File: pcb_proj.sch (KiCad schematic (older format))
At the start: 11 parts, among them U0 OPA333xxDBV, U1 OPA333xxDBV, U2 OPA333xxDBV, U3 OPA333xxDBV, U4 OPA333xxDBV, U5 OPA333xxDBV, U6 OPA333xxDBV, U7 OPA333xxDBV, U8 OPA333xxDBV, U9 OPA333xxDBV

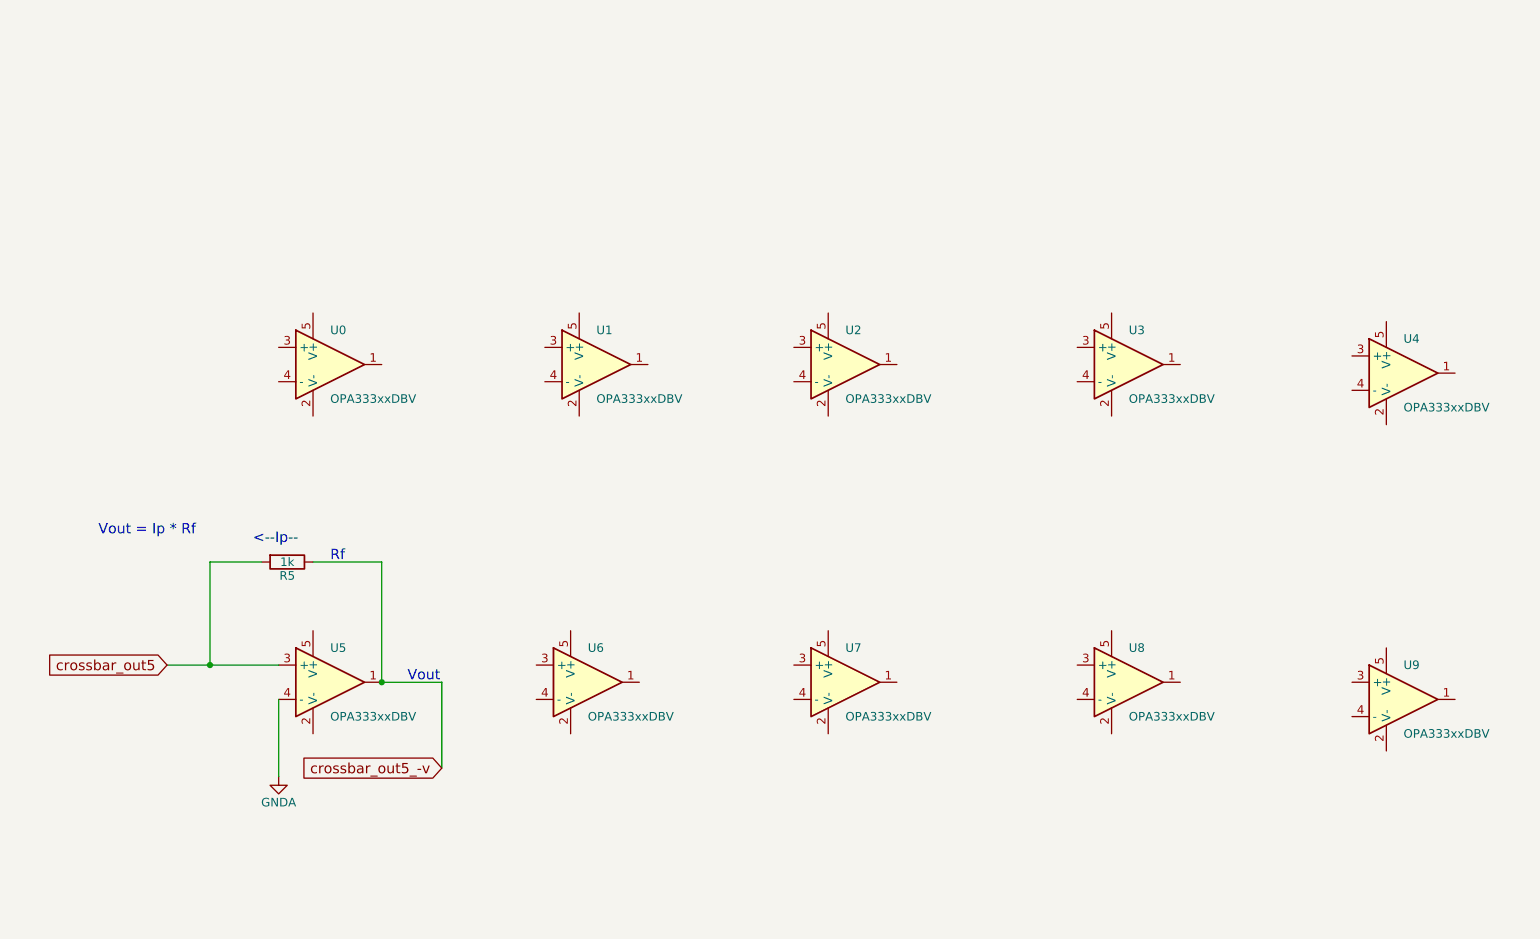
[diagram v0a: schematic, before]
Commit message: About to make a heirarchy, committing first in case we need to go back
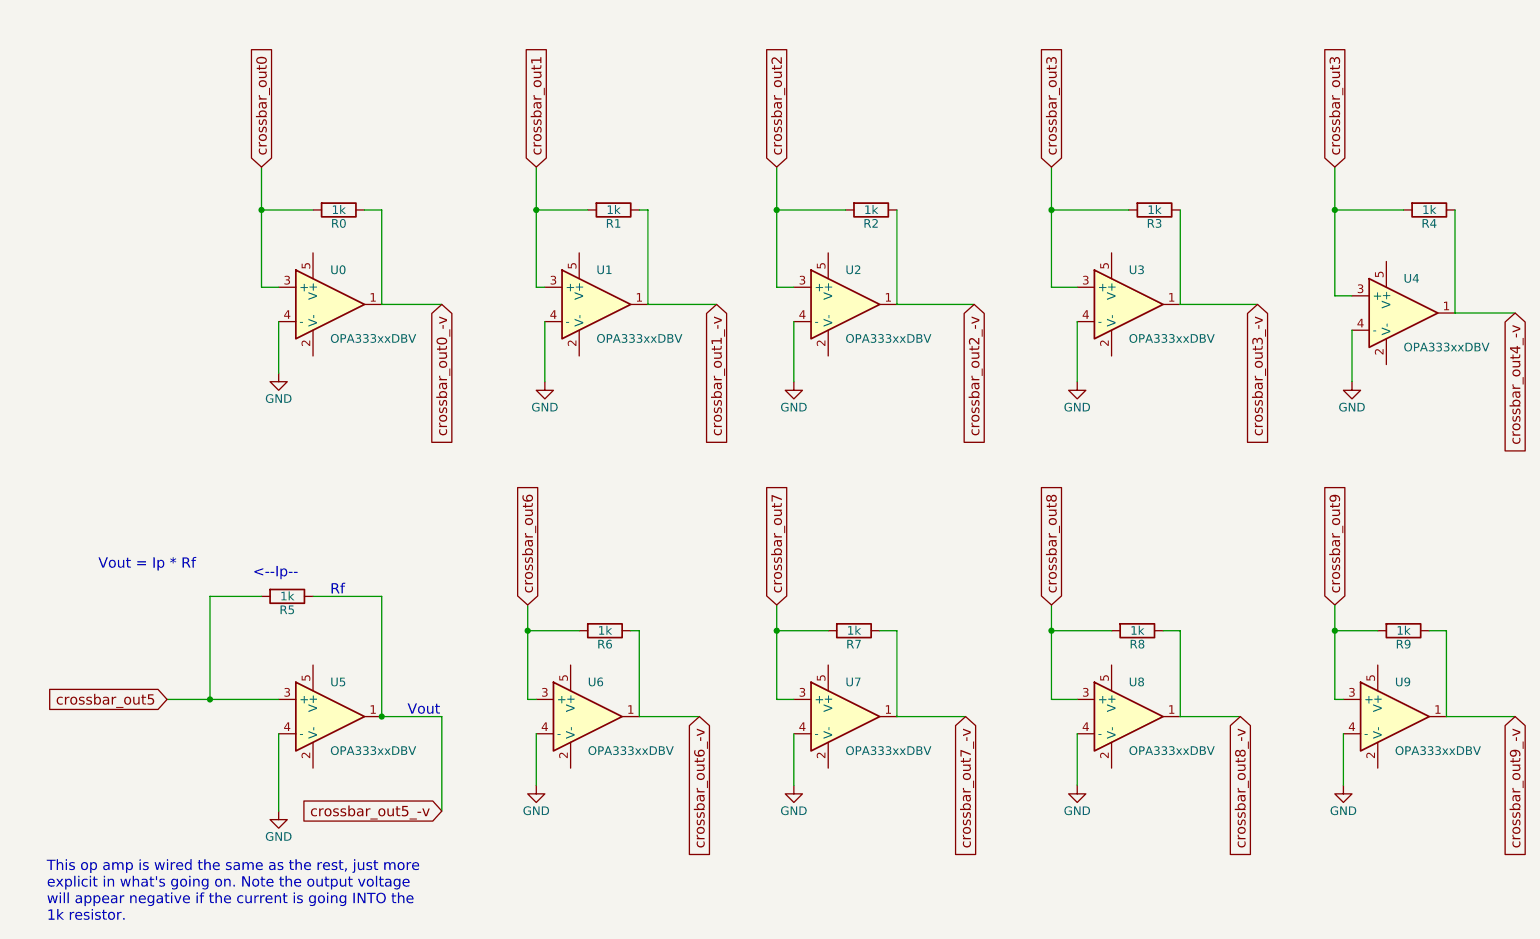
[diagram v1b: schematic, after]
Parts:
- added R0, R1, R2, R3, R4, R6, R7, R8, R9: 1k, symbol R
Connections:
- net GNDA is gone; now on net GND: U5.4 (-)
- net crossbar_out4_-v: now reaches U4.1
- net crossbar_out4_-v: now also R4.1
- net crossbar_out3: now reaches U4.3 (+)
- net crossbar_out3: now also U3.3 (+), R3.2, R4.2
- net GND: now reaches U4.4 (-)
- net GND: now also U0.4 (-), U1.4 (-), U2.4 (-), U3.4 (-), U6.4 (-), U7.4 (-), U8.4 (-), U9.4 (-)
- net crossbar_out7_-v: now reaches U7.1
- net crossbar_out7_-v: now also R7.1
- net crossbar_out7: now reaches U7.3 (+)
- net crossbar_out7: now also R7.2
- net crossbar_out9_-v: now reaches U9.1
- net crossbar_out9_-v: now also R9.1
- net crossbar_out9: now reaches U9.3 (+)
- net crossbar_out9: now also R9.2
- net crossbar_out2_-v: now reaches U2.1
- net crossbar_out2_-v: now also R2.1
- net crossbar_out2: now reaches U2.3 (+)
- net crossbar_out2: now also R2.2
- net crossbar_out3_-v: now reaches U3.1
- net crossbar_out3_-v: now also R3.1
- net crossbar_out6_-v: now reaches U6.1
- net crossbar_out6_-v: now also R6.1
- net crossbar_out6: now reaches U6.3 (+)
- net crossbar_out6: now also R6.2
- net crossbar_out8_-v: now reaches U8.1
- net crossbar_out8_-v: now also R8.1
- net crossbar_out8: now reaches U8.3 (+)
- net crossbar_out8: now also R8.2
- net crossbar_out1_-v: now reaches U1.1
- net crossbar_out1_-v: now also R1.1
- net crossbar_out1: now reaches U1.3 (+)
- net crossbar_out1: now also R1.2
- net crossbar_out0_-v: now reaches U0.1
- net crossbar_out0_-v: now also R0.1
- net crossbar_out0: now reaches U0.3 (+)
- net crossbar_out0: now also R0.2
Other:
- note added: "This op amp is wired the same as the rest, just more\nexplicit in what's going on. Note the output voltage \nwill appear negative if the current is going INTO the \n1k resistor."
- moved on the sheet: R5, U0, U1, U2, U3, U4, U5, U6, U7, U8, U9
